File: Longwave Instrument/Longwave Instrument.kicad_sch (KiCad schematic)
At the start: 34 parts, among them U8 ADR510, U9 ADR510

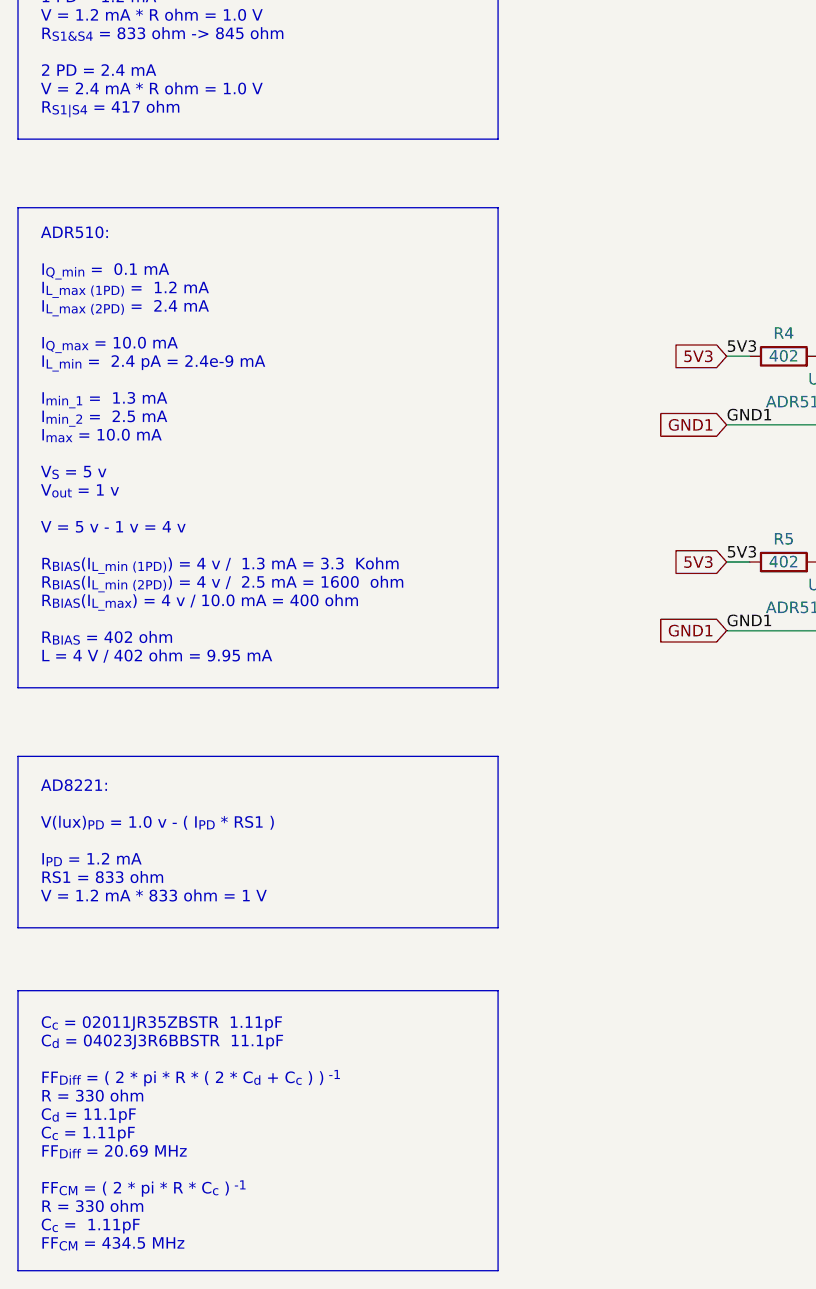
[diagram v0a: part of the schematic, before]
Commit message: SpectDrone Development
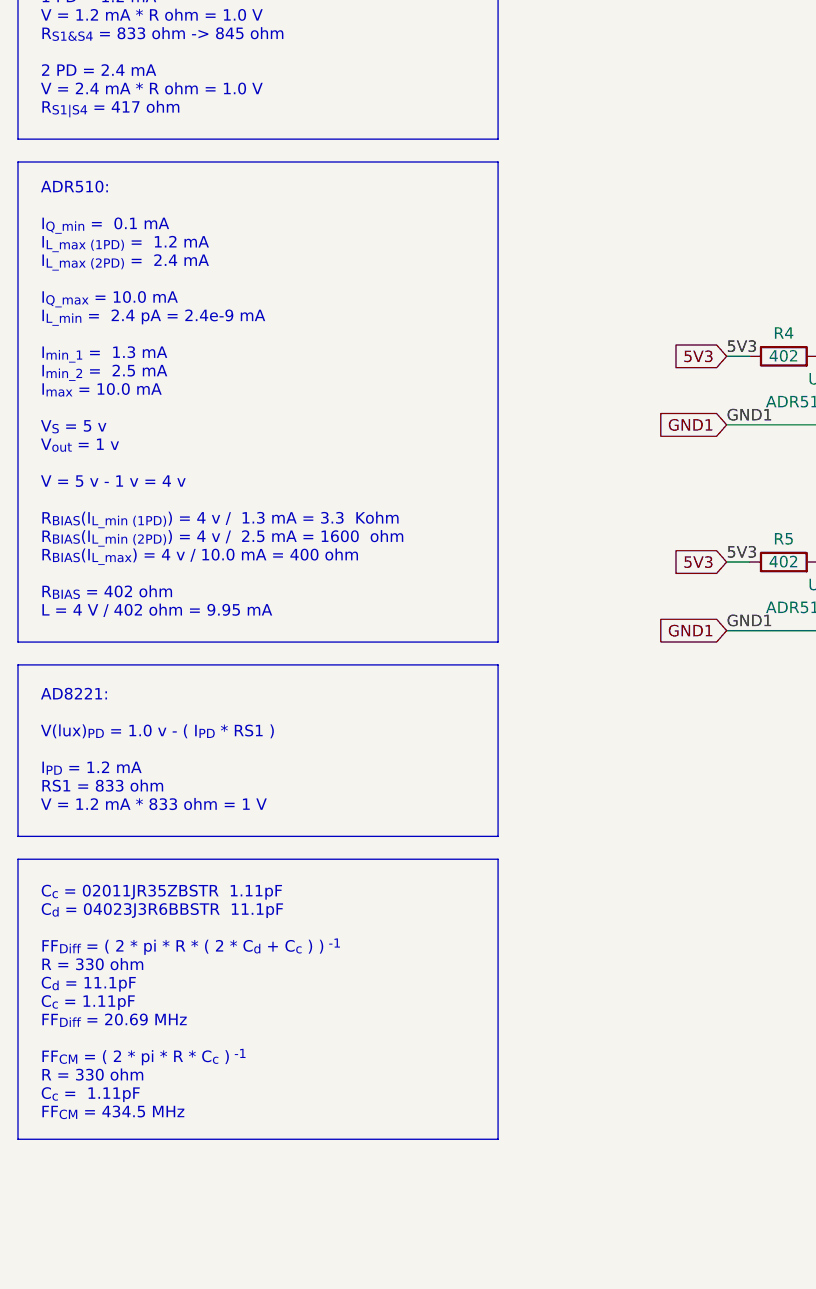
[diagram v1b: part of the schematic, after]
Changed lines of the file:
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@@
     (stroke (width 0) (type default) (color 0 0 0 0))
   )
-  (polyline (pts (xy 67.31 128.27) (xy 67.31 147.32))
+  (polyline (pts (xy 67.31 118.11) (xy 67.31 137.16))
     (stroke (width 0) (type default) (color 0 0 0 0))
   )
@@
     (stroke (width 0) (type default) (color 0 0 0 0))
   )
-  (polyline (pts (xy 13.97 67.31) (xy 67.31 67.31))
+  (polyline (pts (xy 13.97 62.23) (xy 67.31 62.23))
     (stroke (width 0) (type default) (color 0 0 0 0))
   )
@@
     (stroke (width 0) (type default) (color 0 0 0 0))
   )
-  (polyline (pts (xy 67.31 67.31) (xy 67.31 120.65))
+  (polyline (pts (xy 67.31 62.23) (xy 67.31 115.57))
     (stroke (width 0) (type default) (color 0 0 0 0))
   )
@@
     (stroke (width 0) (type default) (color 0 0 0 0))
   )
-  (polyline (pts (xy 67.31 185.42) (xy 13.97 185.42))
+  (polyline (pts (xy 67.31 170.815) (xy 13.97 170.815))
     (stroke (width 0) (type default) (color 0 0 0 0))
   )
@@
     (stroke (width 0) (type default) (color 0 0 0 0))
   )
-  (polyline (pts (xy 67.31 147.32) (xy 13.97 147.32))
+  (polyline (pts (xy 67.31 137.16) (xy 13.97 137.16))
     (stroke (width 0) (type default) (color 0 0 0 0))
   )
@@
     (stroke (width 0) (type default) (color 0 0 0 0))
   )
-  (polyline (pts (xy 67.31 120.65) (xy 13.97 120.65))
+  (polyline (pts (xy 67.31 115.57) (xy 13.97 115.57))
     (stroke (width 0) (type default) (color 0 0 0 0))
   )
@@
     (stroke (width 0) (type default) (color 0 0 0 0))
   )
-  (polyline (pts (xy 67.31 154.305) (xy 67.31 185.42))
+  (polyline (pts (xy 67.31 139.7) (xy 67.31 170.815))
     (stroke (width 0) (type default) (color 0 0 0 0))
   )
@@
     (stroke (width 0) (type default) (color 0 0 0 0))
   )
-  (polyline (pts (xy 13.97 128.27) (xy 67.31 128.27))
+  (polyline (pts (xy 13.97 118.11) (xy 67.31 118.11))
     (stroke (width 0) (type default) (color 0 0 0 0))
   )
@@
     (stroke (width 0) (type default) (color 0 0 0 0))
   )
-  (polyline (pts (xy 13.97 154.305) (xy 67.31 154.305))
+  (polyline (pts (xy 13.97 139.7) (xy 67.31 139.7))
     (stroke (width 0) (type default) (color 0 0 0 0))
   )
@@
     (stroke (width 0) (type default) (color 0 0 0 0))
   )
-  (polyline (pts (xy 13.97 185.42) (xy 13.97 154.305))
+  (polyline (pts (xy 13.97 170.815) (xy 13.97 139.7))
     (stroke (width 0) (type default) (color 0 0 0 0))
   )
@@
     (stroke (width 0) (type default) (color 0 0 0 0))
   )
-  (polyline (pts (xy 13.97 147.32) (xy 13.97 128.27))
+  (polyline (pts (xy 13.97 137.16) (xy 13.97 118.11))
     (stroke (width 0) (type default) (color 0 0 0 0))
   )
@@
     (stroke (width 0) (type default) (color 0 0 0 0))
   )
-  (polyline (pts (xy 13.97 120.65) (xy 13.97 67.31))
+  (polyline (pts (xy 13.97 115.57) (xy 13.97 62.23))
     (stroke (width 0) (type default) (color 0 0 0 0))
   )
@@
   )
   (text "C_{c} = 02011JR35ZBSTR  1.11pF\nC_{d} = 04023J3R6BBSTR  11.1pF\n\nFF_{Diff} = ( 2 * pi * R * ( 2 * C_{d} + C_{c} ) )^{ -1}\nR = 330 ohm\nC_{d} = 11.1pF\nC_{c} = 1.11pF\nFF_{Diff} = 20.69 MHz\n\nFF_{CM} = ( 2 * pi * R * C_{c} )^{ -1}\nR = 330 ohm\nC_{c} =  1.11pF\nFF_{CM} = 434.5 MHz\n\n"
-    (at 16.51 185.42 0)
+    (at 16.51 170.815 0)
     (effects (font (size 1.27 1.27)) (justify left bottom))
   )
   (text "ADR510:\n\nI_{Q_min} =  0.1 mA\nI_{L_max (1PD)} =  1.2 mA\nI_{L_max (2PD)} =  2.4 mA\n\nI_{Q_max} = 10.0 mA\nI_{L_min} =  2.4 pA = 2.4e-9 mA\n\nI_{min_1} =  1.3 mA\nI_{min_2} =  2.5 mA\nI_{max} = 10.0 mA\n\nV_{S} = 5 v\nV_{out} = 1 v\n\nV = 5 v - 1 v = 4 v\n\nR_{BIAS}(I_{L_min (1PD)}) = 4 v /  1.3 mA = 3.3  Kohm\nR_{BIAS}(I_{L_min (2PD)}) = 4 v /  2.5 mA = 1600  ohm\nR_{BIAS}(I_{L_max}) = 4 v / 10.0 mA = 400 ohm\n\nR_{BIAS} = 402 ohm\nL = 4 V / 402 ohm = 9.95 mA"
-    (at 16.51 118.11 0)
+    (at 16.51 113.03 0)
     (effects (font (size 1.27 1.27)) (justify left bottom))
   )
   (text "AD8221:\n\nV(lux)_{PD} = 1.0 v - ( I_{PD} * RS1 )\n\nI_{PD} = 1.2 mA\nRS1 = 833 ohm\nV = 1.2 mA * 833 ohm = 1 V"
-    (at 16.51 144.78 0)
+    (at 16.51 134.62 0)
     (effects (font (size 1.27 1.27)) (justify left bottom))
   )

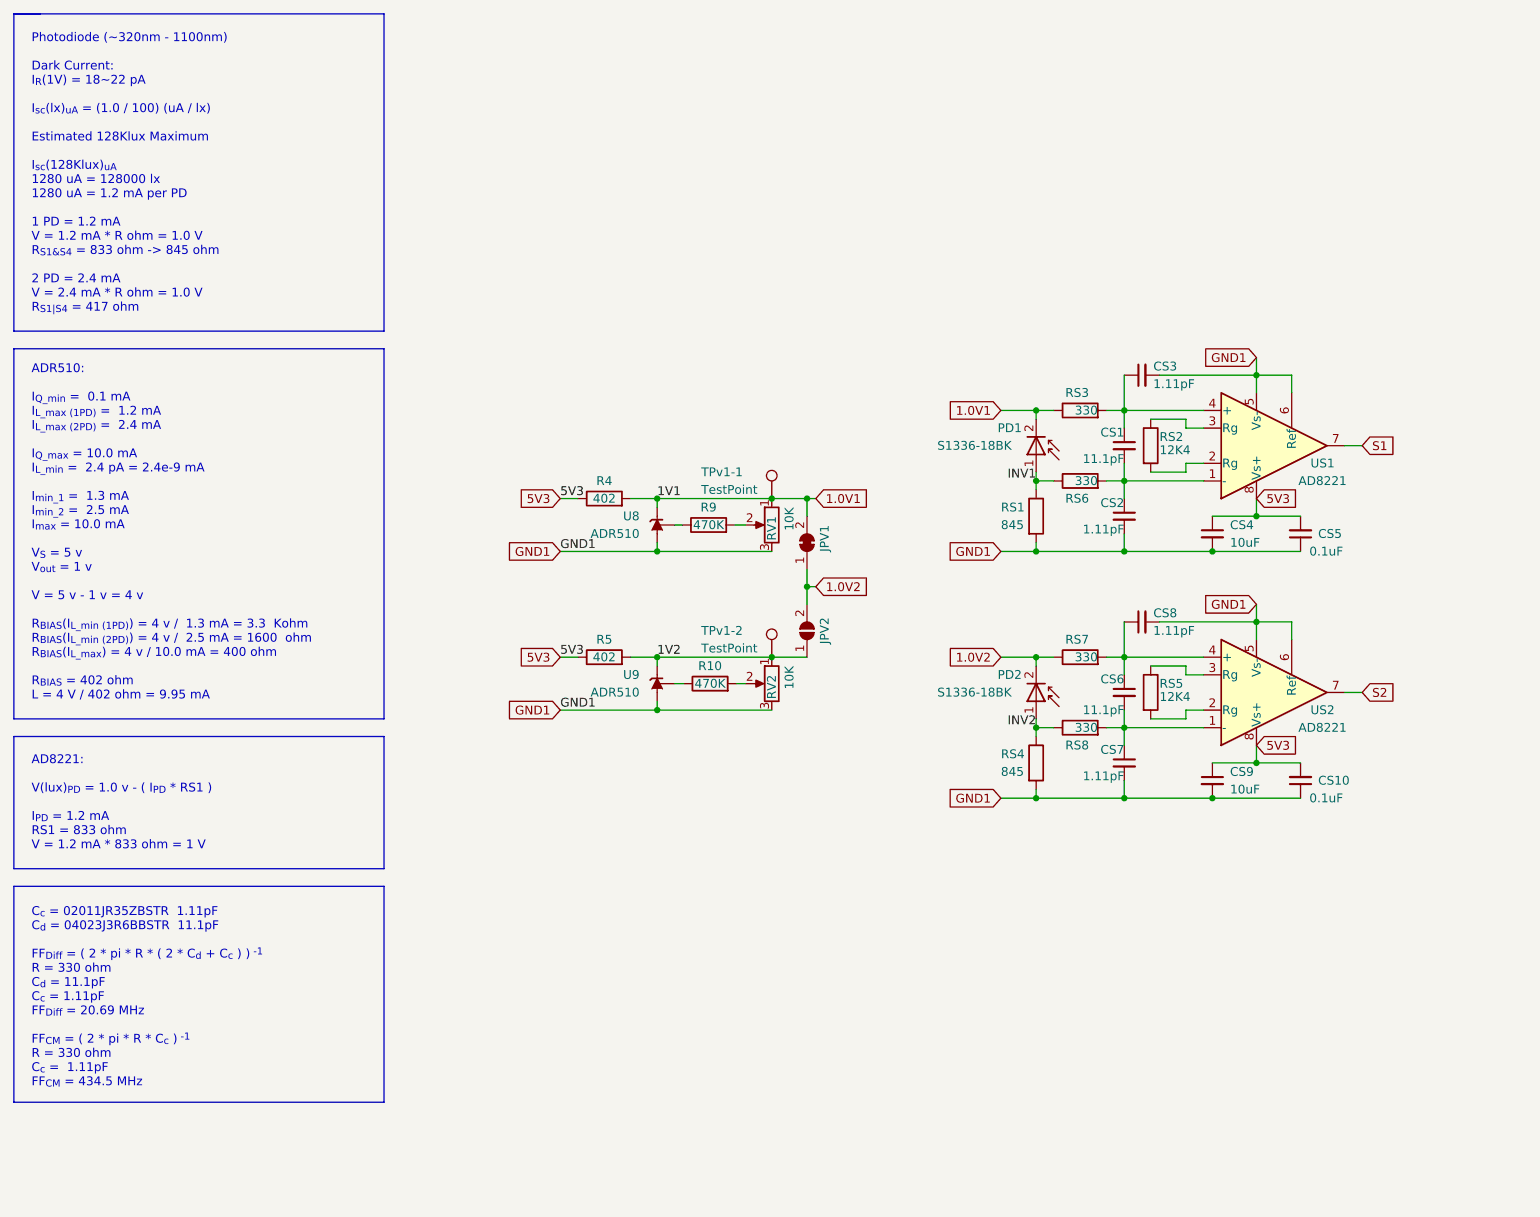
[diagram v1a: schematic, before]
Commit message: SpectDrone Development
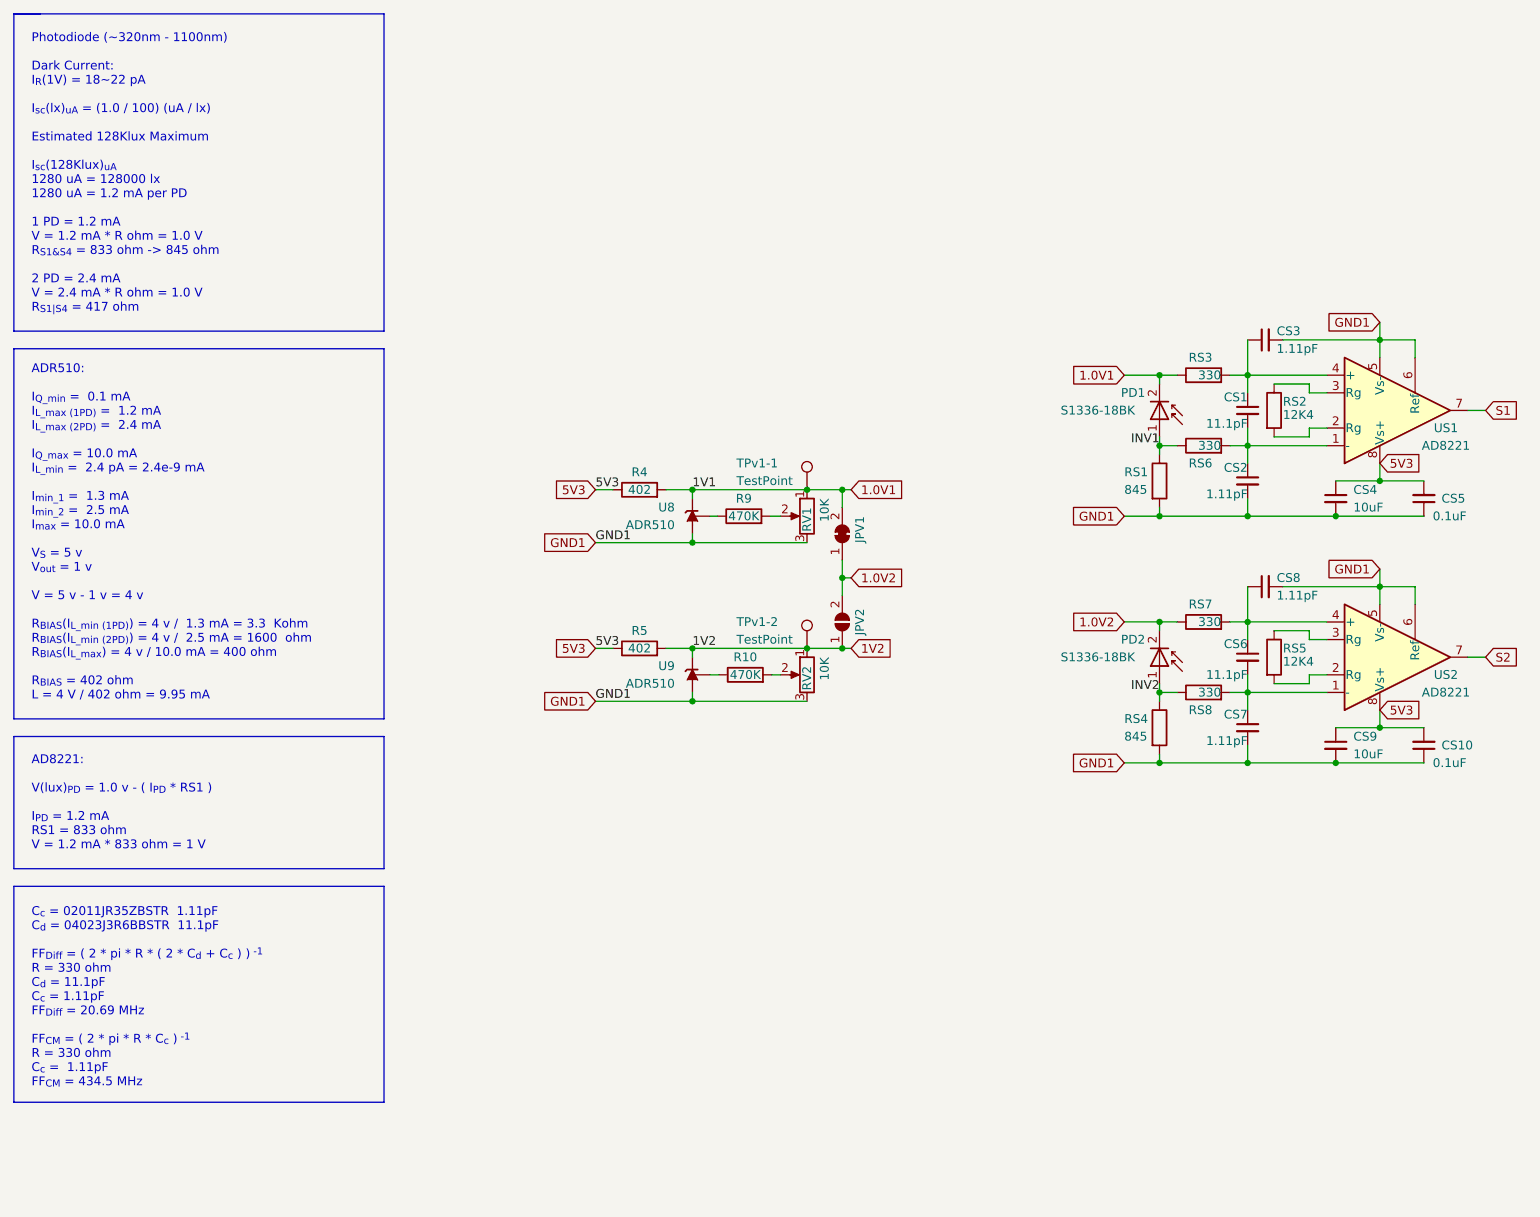
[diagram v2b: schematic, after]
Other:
- moved on the sheet: CS1, CS10, CS2, CS3, CS4, CS5, CS6, CS7, CS8, CS9, JPV1, JPV2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

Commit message: SpectDrone Development
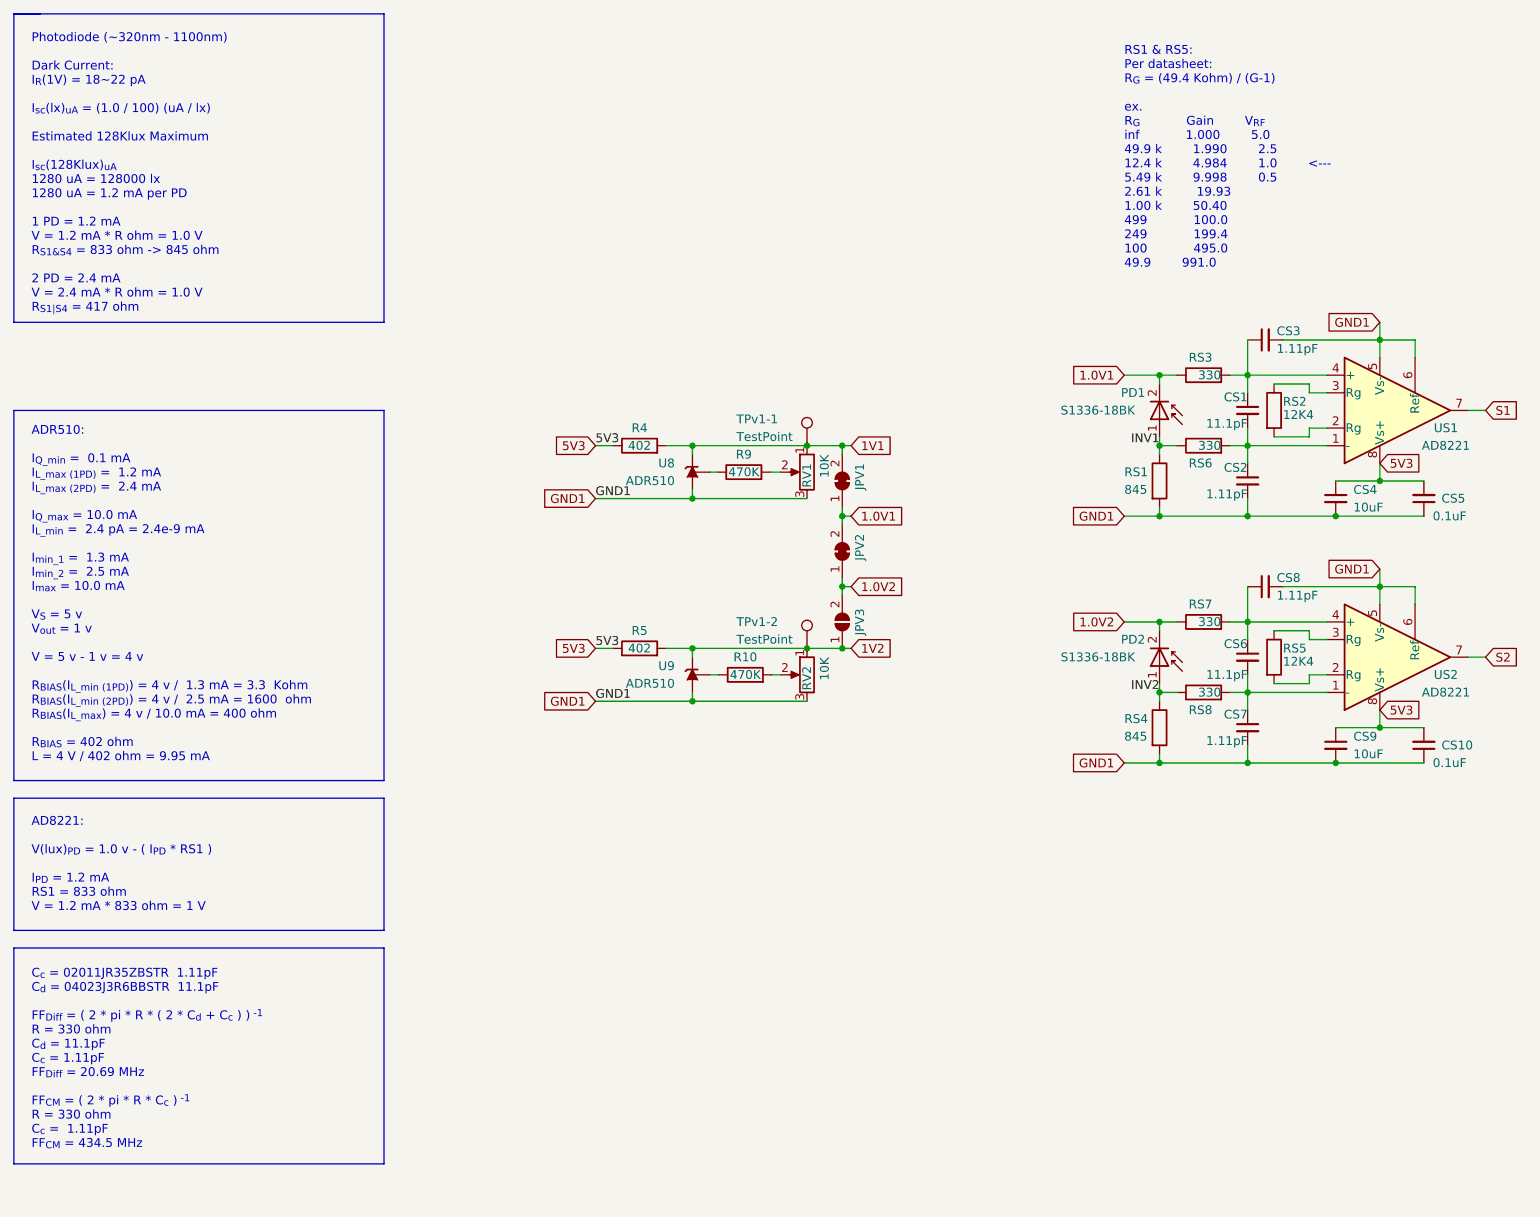
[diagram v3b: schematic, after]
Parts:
- added JPV1: SolderJumper_2_Bridged, Jumper:SolderJumper-2_P1.3mm_Bridged_RoundedPad1.0x1.5mm, symbol Jumper:SolderJumper_2_Bridged
- renumbered JPV1 to JPV2, JPV2 to JPV3
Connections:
- net 1.0V1: now also JPV1.1 (A); no longer R4.2, RV1.1, TPv1-1.1, U8.2 (K)
- new net 1V1: JPV1.2 (B), R4.2, RV1.1, TPv1-1.1, U8.2 (K)
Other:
- note added: "RS1 & RS5: Per datasheet: R_{G} = (49.4 Kohm) / (G-1) ex. R_{G} Gain V_{RF} inf 1.000 5.0 49.9 k 1.990 2.5 12.4 k 4.984 1.0 <--- 5.49 k 9.998 0.5 2.61 k 19.93 1.00 k 50.40 499 100.0 249 199.4 100 495.0 49.9 991.0"
- moved on the sheet: JPV2, R4, R9, RV1, TPv1-1, U8
